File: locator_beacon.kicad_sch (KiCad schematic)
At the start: 1 part

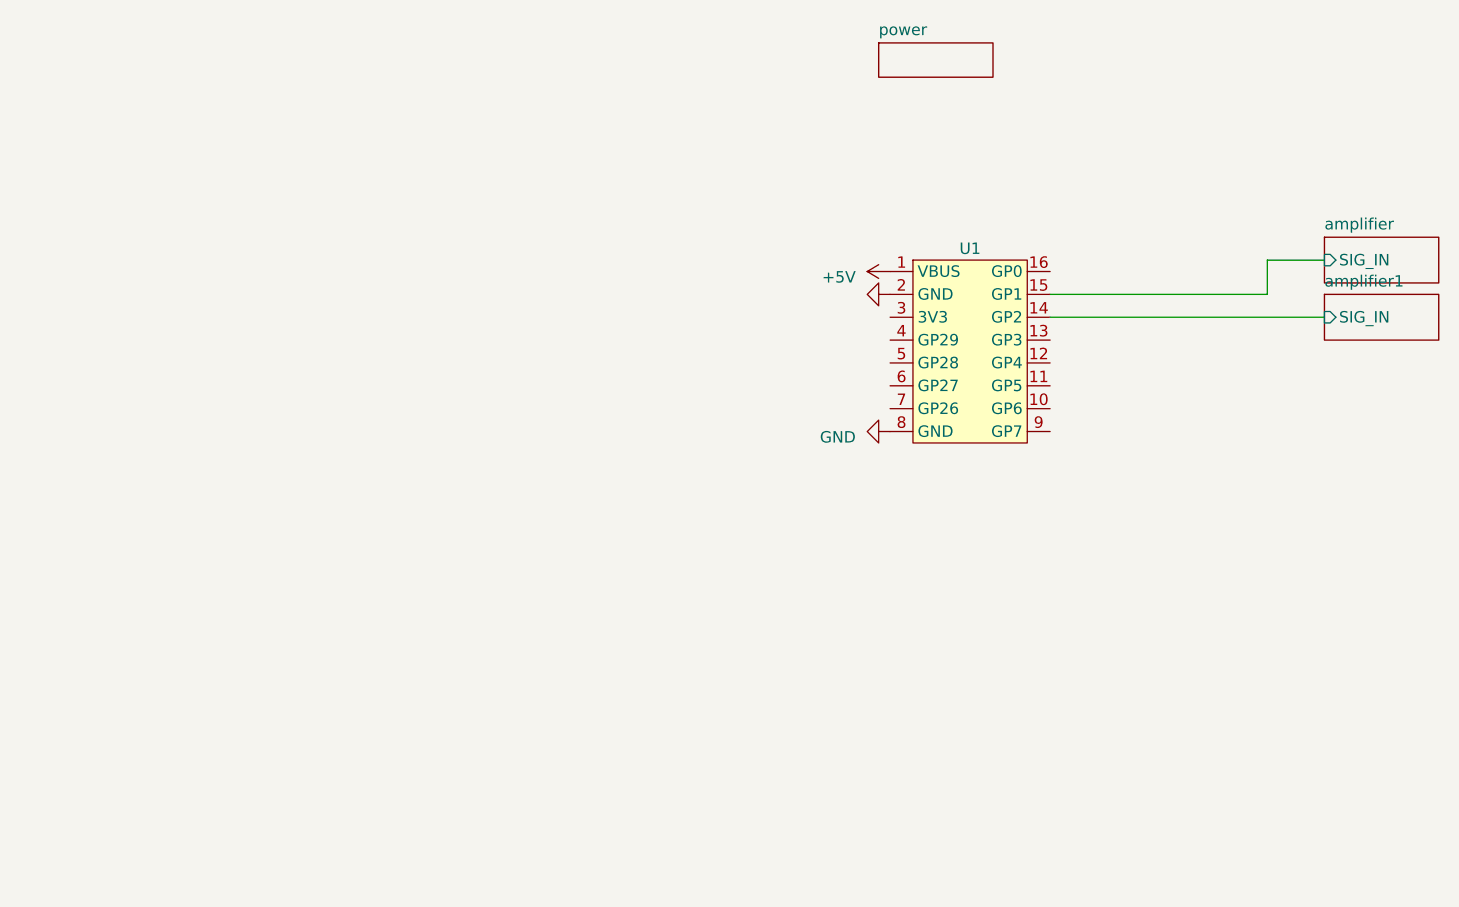
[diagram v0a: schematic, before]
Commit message: Seems reasonable
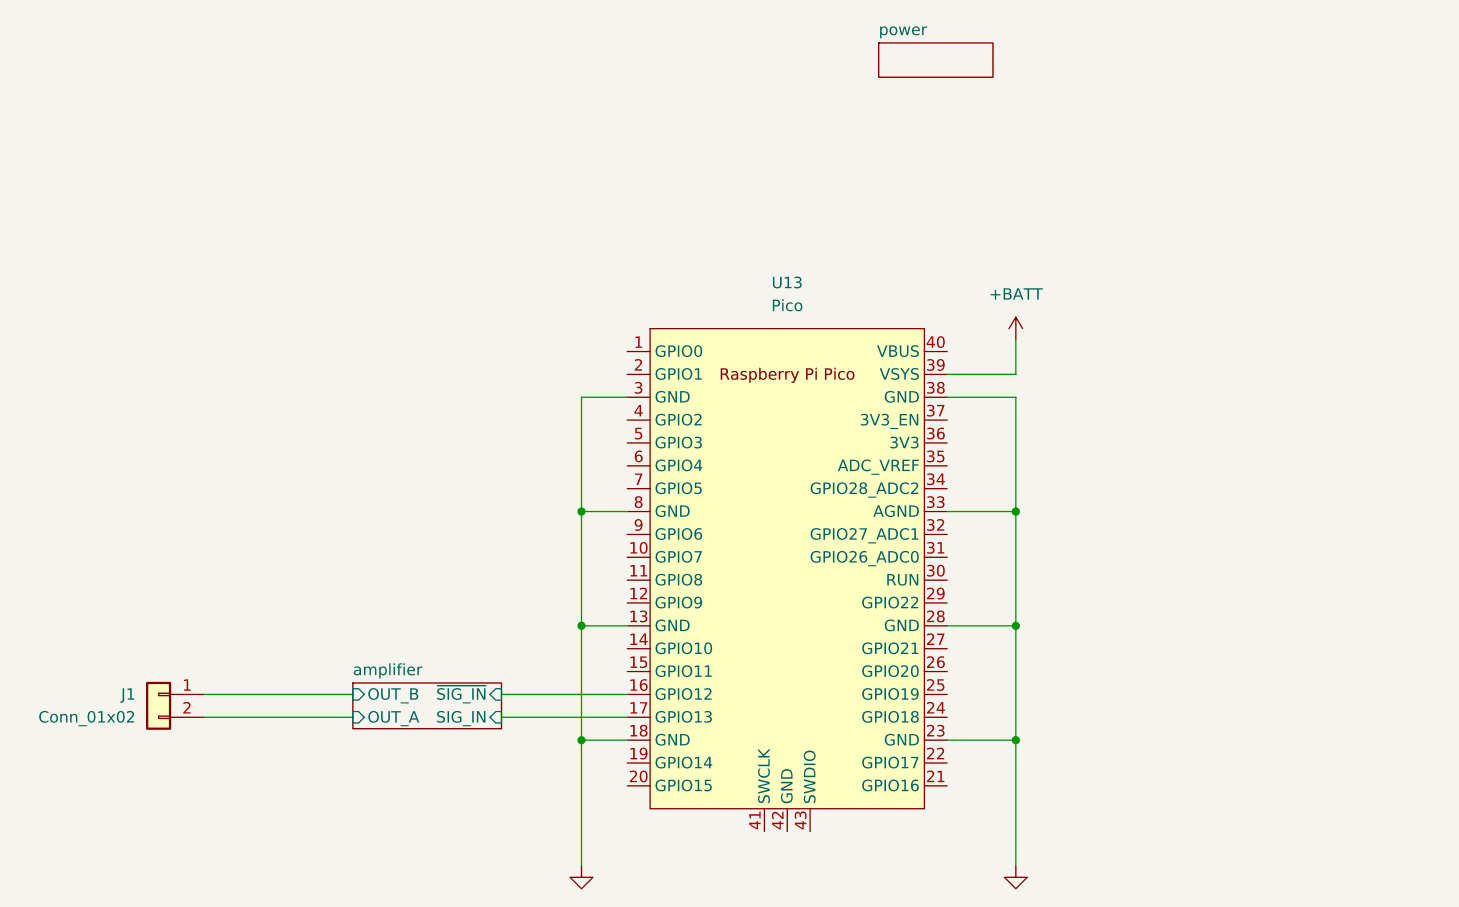
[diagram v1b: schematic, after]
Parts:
- removed U1: ~, RPi:tiny_2040, symbol custom_symbols:tiny_2040
- added J1: Conn_01x02, Connector_PinHeader_2.54mm:PinHeader_1x02_P2.54mm_Horizontal, symbol Connector_Generic:Conn_01x02
- added U13: Pico, custom:rp_pico, symbol MCU_RaspberryPi_and_Boards:Pico
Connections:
- net GND: now also U13.13 (GND), U13.18 (GND), U13.23 (GND), U13.28 (GND), U13.3 (GND), U13.33 (AGND), U13.38 (GND), U13.8 (GND)
- net amplifier/SIG_IN: now also U13.17 (GPIO13)
- new net +BATT: U13.39 (VSYS)
- new net amplifier/OUT_A: J1.2 (Pin_2)
- new net amplifier/OUT_B: J1.1 (Pin_1)
- new net amplifier/~{SIG_IN}: U13.16 (GPIO12)
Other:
- removed sheet amplifier1
- sheet amplifier ports: added OUT_A, OUT_B, ~{SIG_IN}; removed none
